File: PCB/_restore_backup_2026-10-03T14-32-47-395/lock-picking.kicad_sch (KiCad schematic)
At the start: 22 parts, among them U1 HX PZ2.54-1X5P ZZ, U2 DRV8876PWPR, U3 MLX90393SLW-ABA-011-RE, U4 SMTSOM225BTR, U5 S2B-PH-K-S, U6 SMTSOM225BTR, U7 HX TYPE-C 16PIN, U8 AMS1117-5.0_C347223

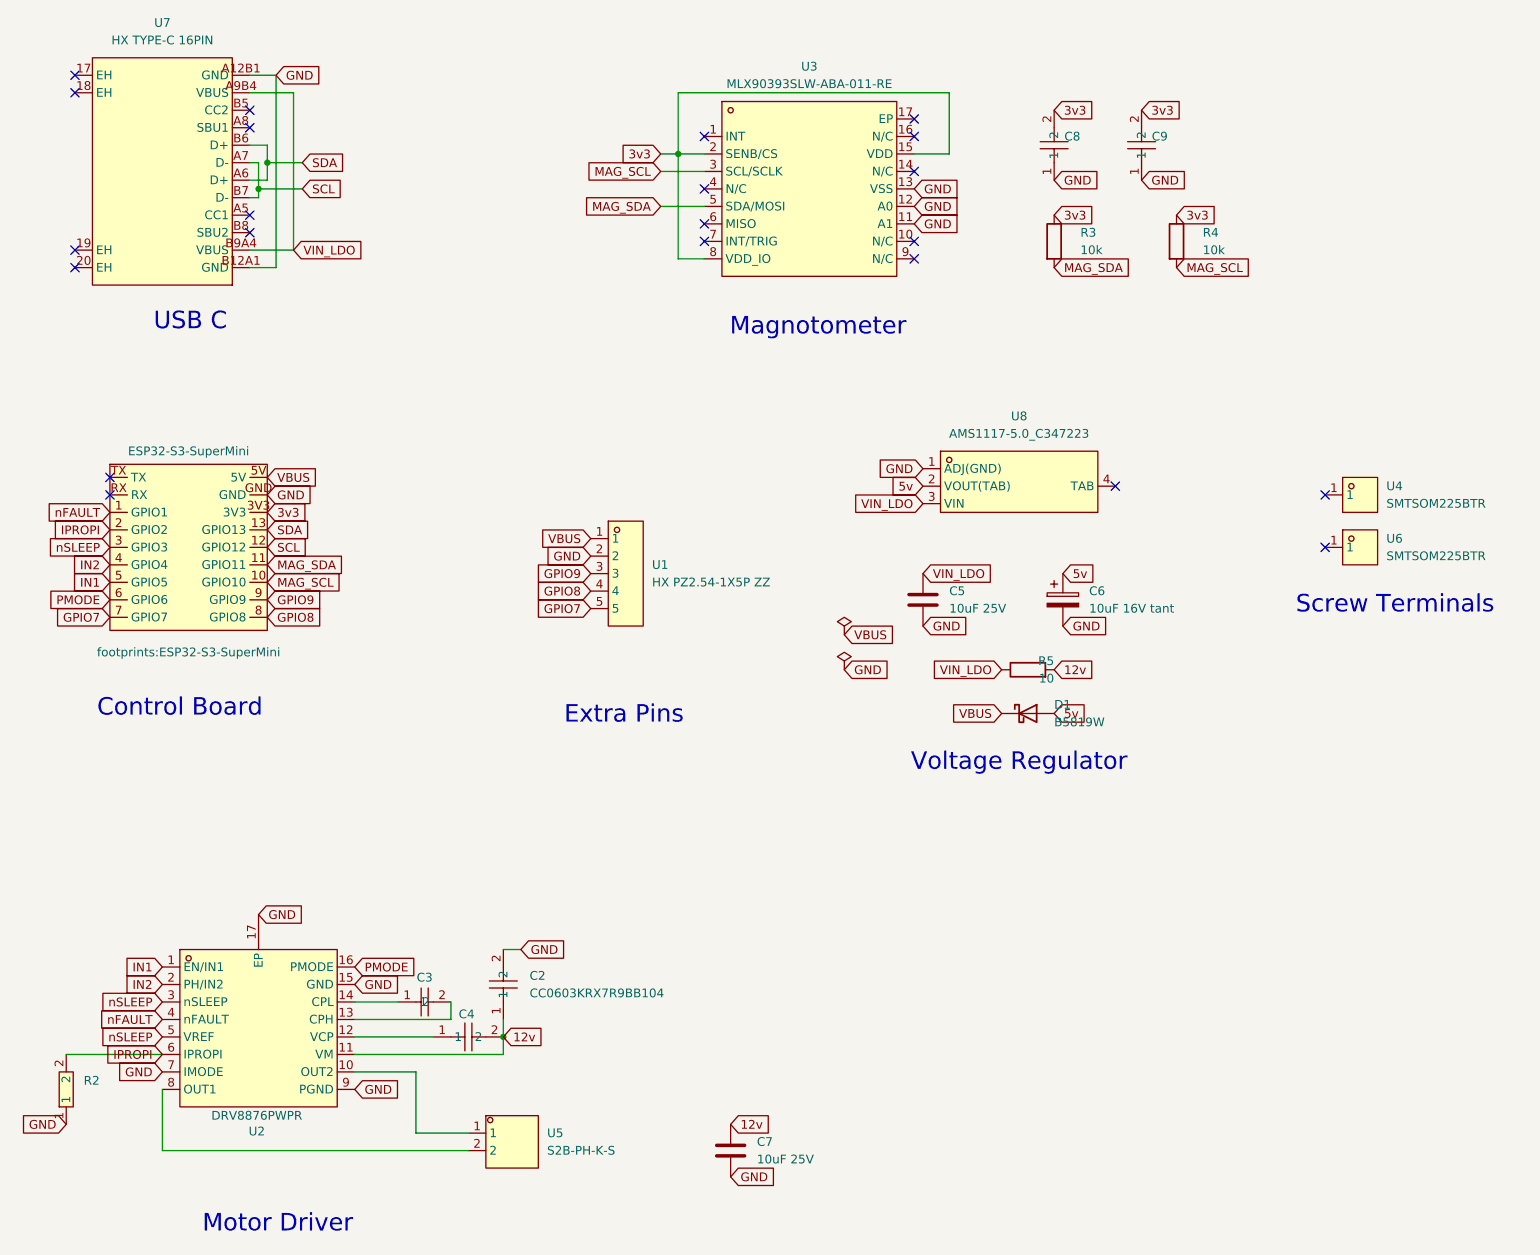
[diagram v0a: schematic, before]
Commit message: PCB updates
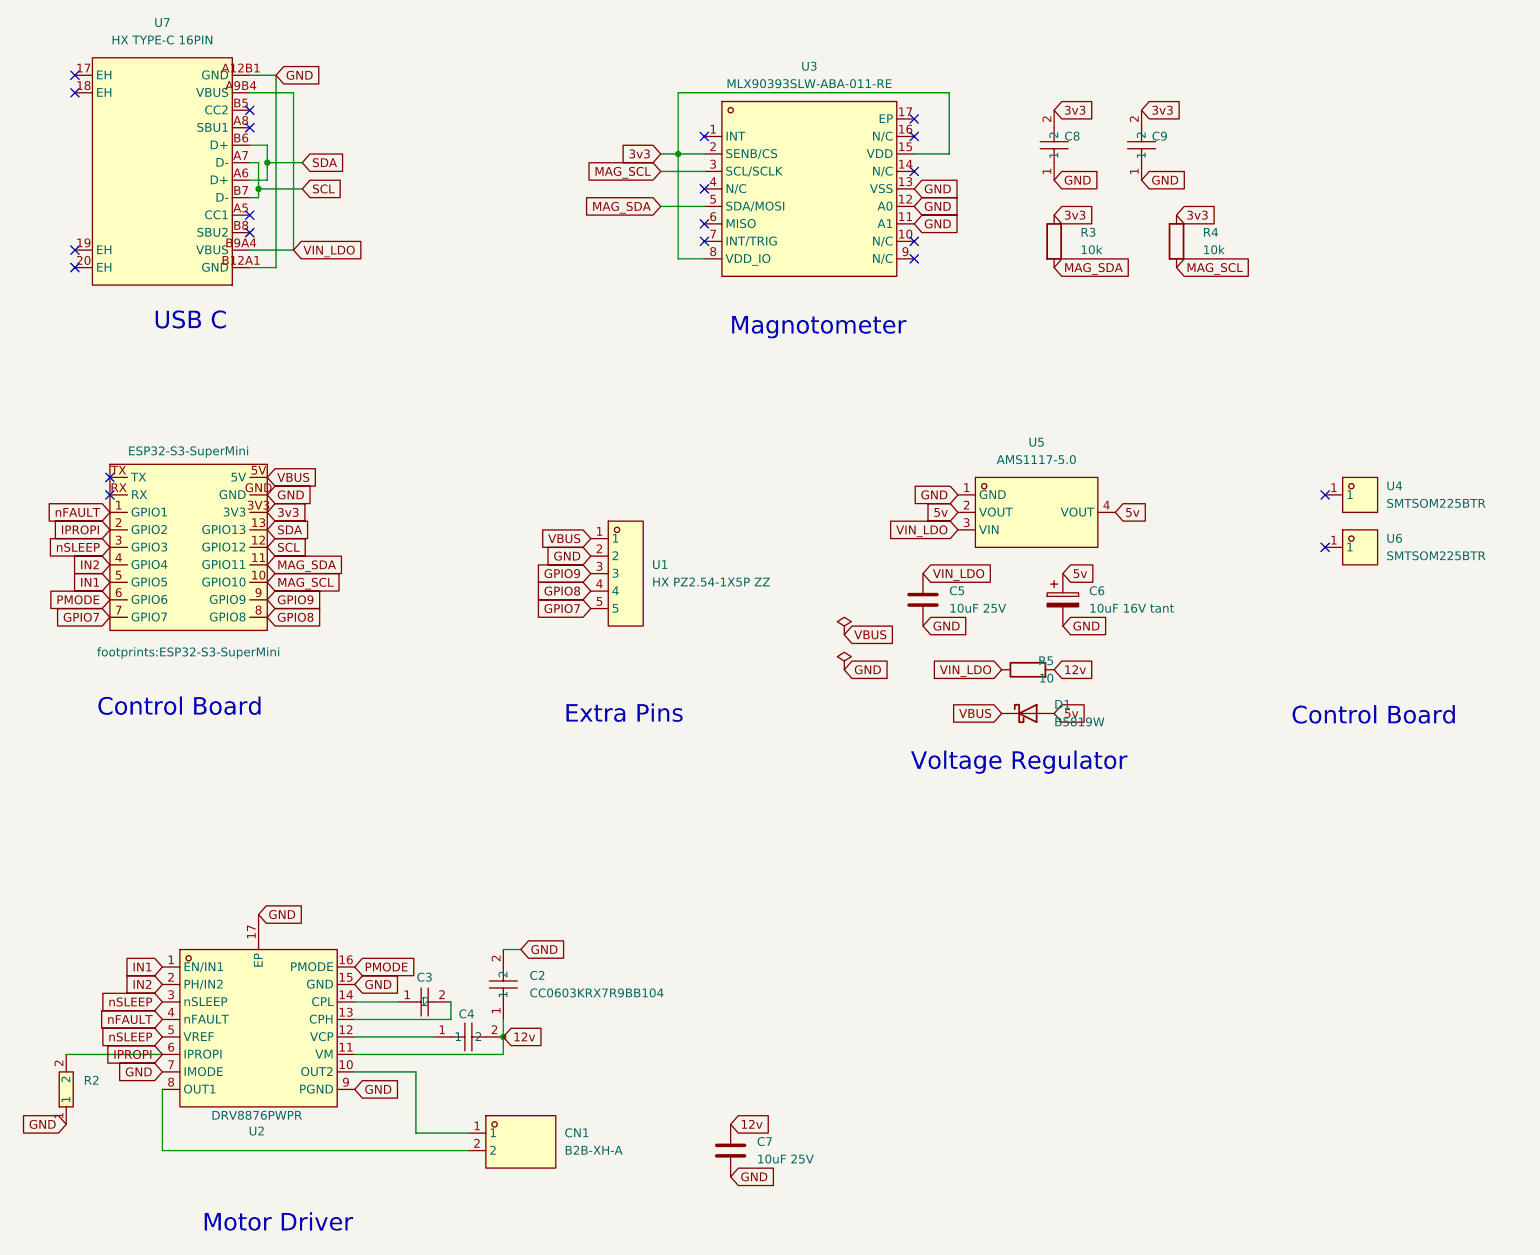
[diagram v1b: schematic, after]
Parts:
- removed U5: S2B-PH-K-S, EasyEDA:CONN-TH_S2B-PH-K-S-LF-SN, symbol EasyEDA:S2B-PH-K-S
- removed U8: AMS1117-5.0_C347223, EasyEDA:SOT-223_L6.7-W3.5-P2.30-BR, symbol EasyEDA:AMS1117-5.0_C347223
- added CN1: B2B-XH-A, EasyEDA:CONN-TH_B2B-XH-A-LF-SN, symbol EasyEDA:B2B-XH-A
- added U5: AMS1117-5.0, EasyEDA:SOT-223_L6.5-W3.5-P2.30-LS7.0-BR, symbol EasyEDA:AMS1117-5.0
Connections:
- net 5v: now also U5.2 (VOUT), U5.4 (VOUT)
- net GND: now also U5.1 (GND)
- net VIN_LDO: now also U5.3 (VIN)
- net at U2.10 (OUT2): now also CN1.1
- net at U2.8 (OUT1): now also CN1.2
- no-connect marks 22 -> 21
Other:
- note removed: "Screw Terminals"
